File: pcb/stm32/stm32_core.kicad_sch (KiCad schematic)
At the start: 21 parts, among them J1 Conn_01x04_Pin, J2 Conn_01x06_Pin, J3 Conn_02x05_Top_Bottom, J4 Conn_01x02_Pin, J5 Conn_02x05_Top_Bottom, J6 Conn_01x02_Pin, SW1 SW_Push, SW2 SW_Push, SW3 SW_Push, U1 STM32G070KBT6

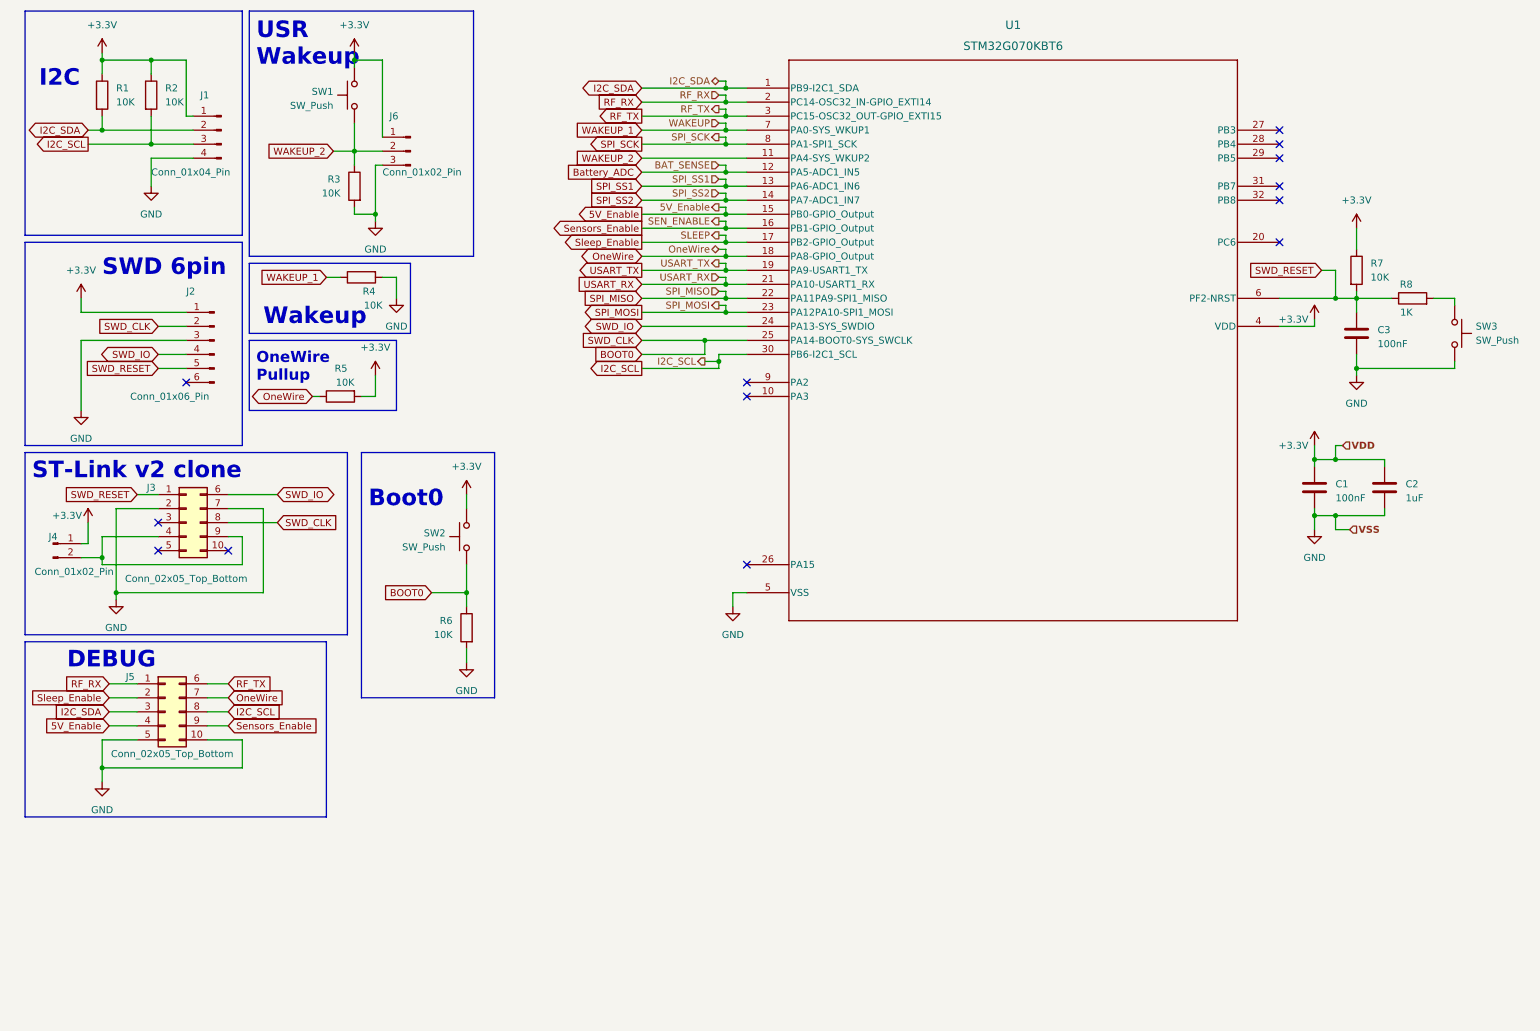
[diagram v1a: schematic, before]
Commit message: Moved PCB forwar
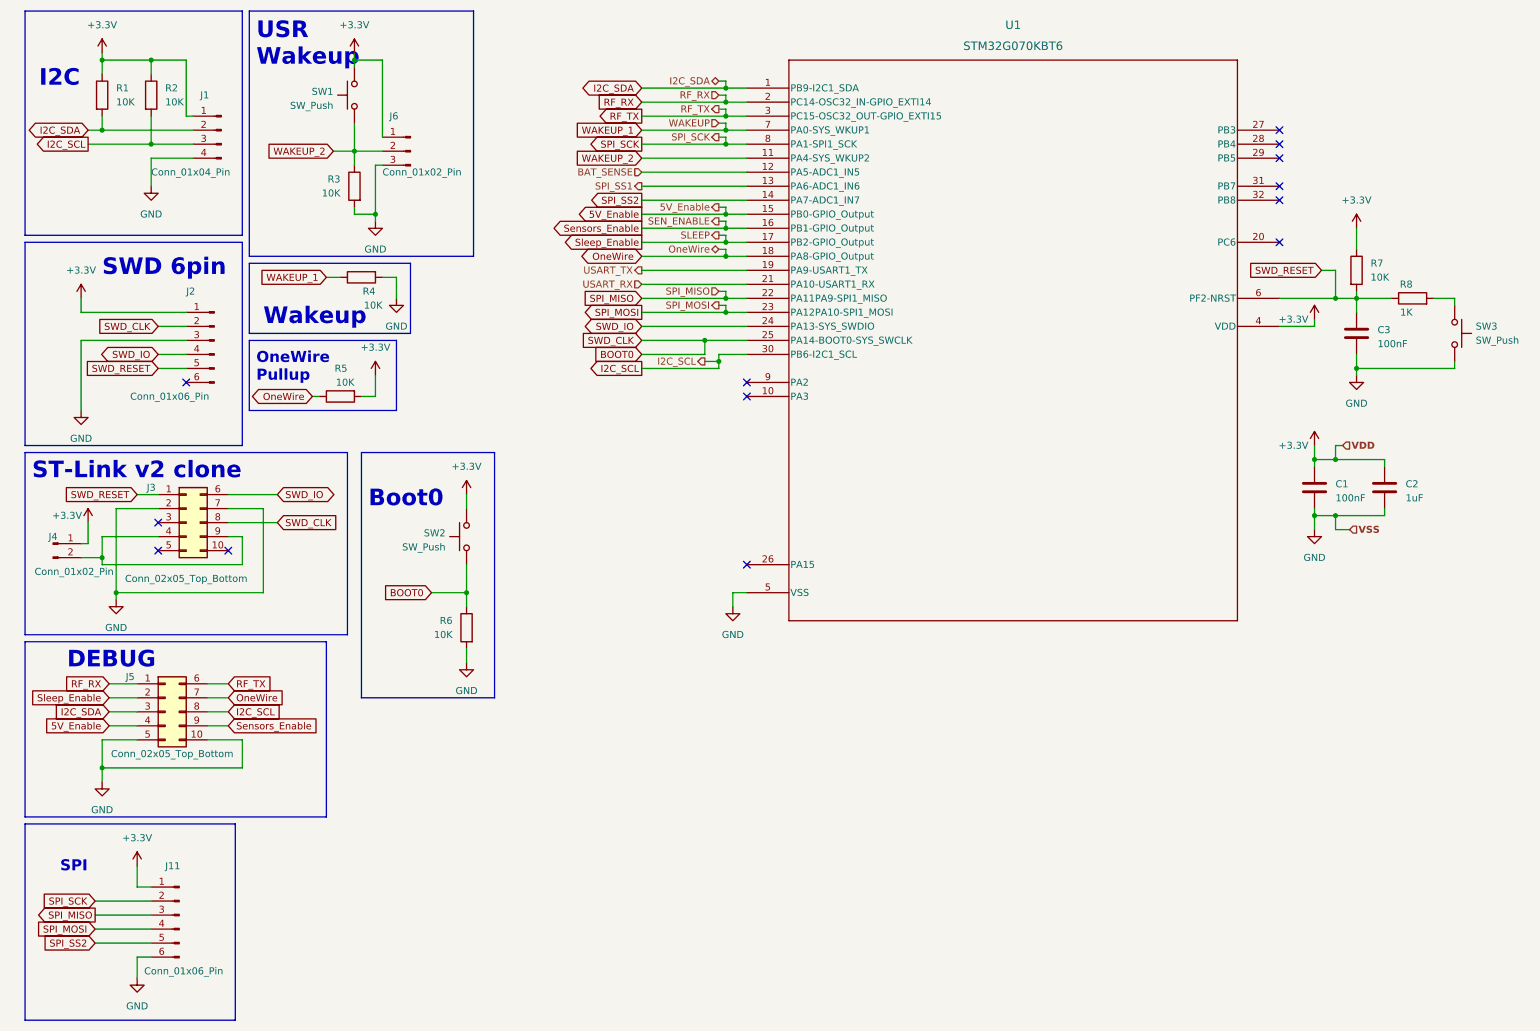
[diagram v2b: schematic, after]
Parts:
- added J11: Conn_01x06_Pin, symbol Connector:Conn_01x06_Pin
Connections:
- net +3.3V: now also J11.1 (Pin_1)
- net GND: now also J11.6 (Pin_6)
- net SPI_MISO: now also J11.3 (Pin_3)
- net SPI_MOSI: now also J11.4 (Pin_4)
- net SPI_SCK: now also J11.2 (Pin_2)
- net SPI_SS2: now also J11.5 (Pin_5)
- net Battery_ADC renamed BAT_SENSE
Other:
- note added: "SPI"
